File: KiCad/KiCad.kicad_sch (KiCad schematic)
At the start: 7 parts, among them J1 LDR, J2 Custom AMUX, J3 Moist Meter, J4 OLED, J5 Servo, U1 NodeMCU1.0(ESP-12E)

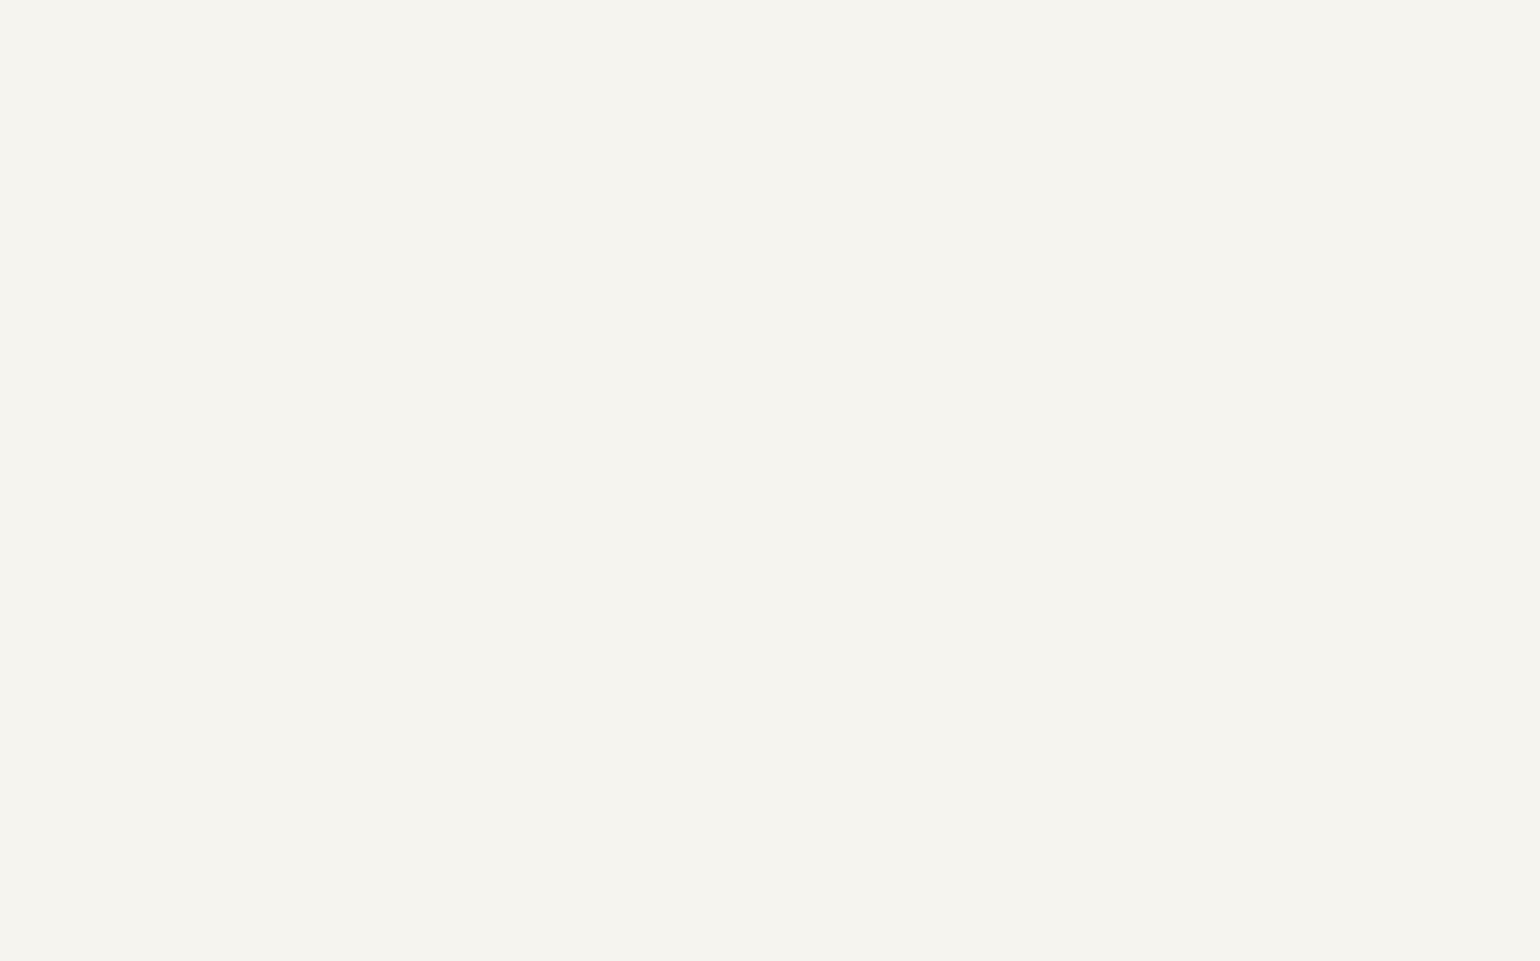
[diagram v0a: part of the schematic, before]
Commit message: kicad
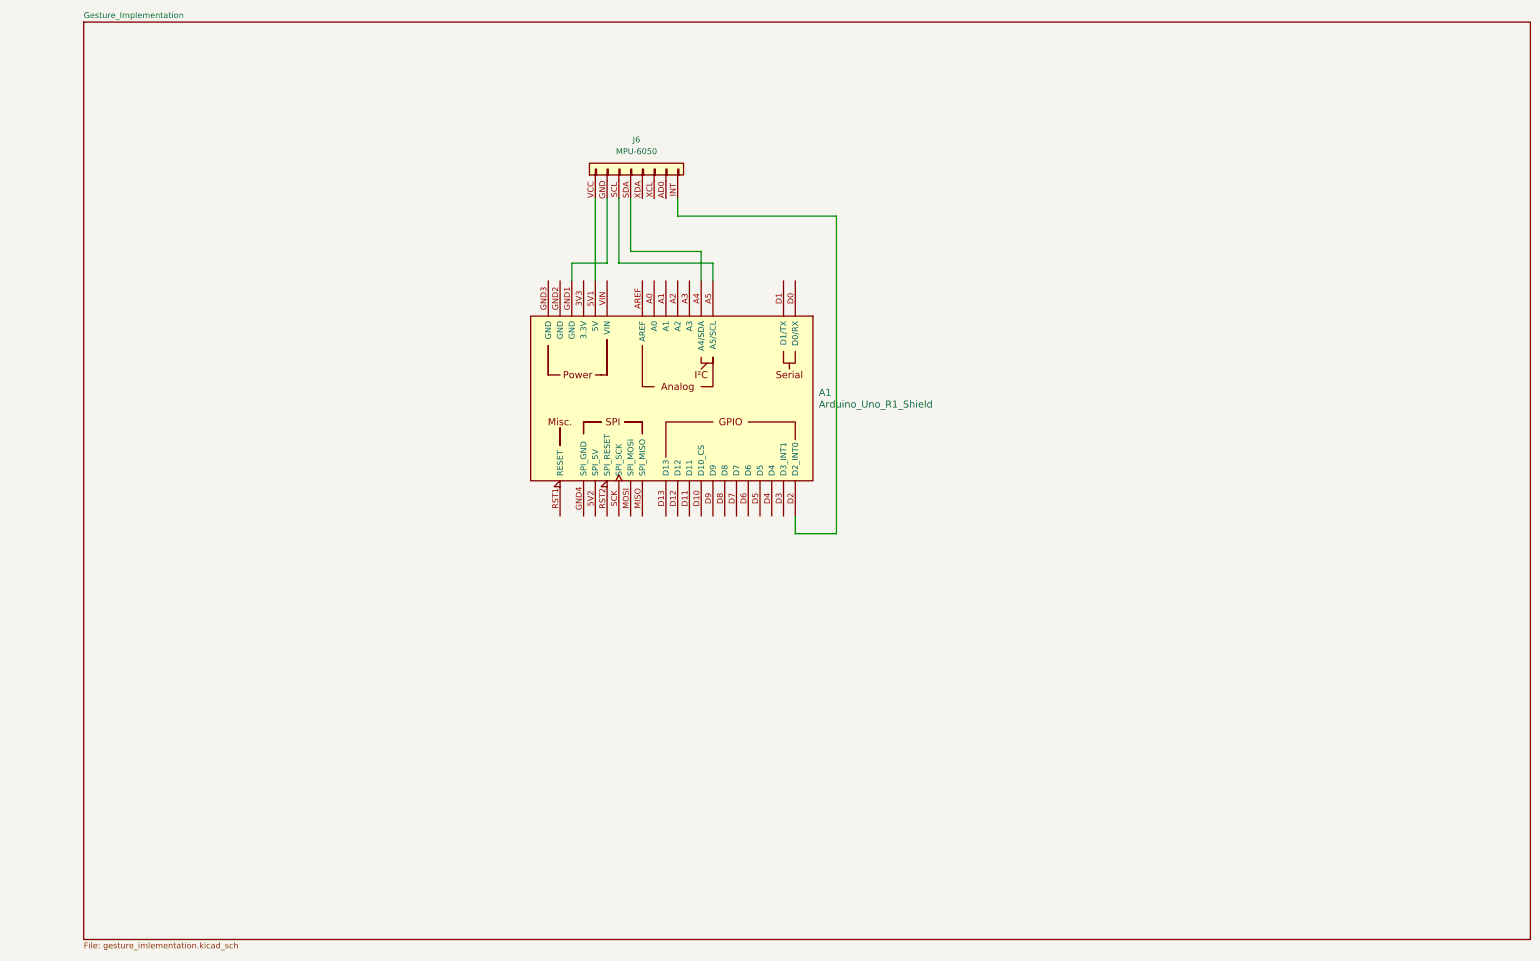
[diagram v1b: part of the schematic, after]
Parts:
- added A1: Arduino_Uno_R1_Shield, PCM_arduino-library:Arduino_Uno_R2_Shield, symbol PCM_arduino-library:Arduino_Uno_R1_Shield
- added J6: MPU-6050, symbol mpu-6050:MPU-6050
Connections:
- new net: A1.GND1 (GND), J6.GND (Pin_2)
- new net: A1.D2 (D2_INT0), J6.INT (8)
- new net: A1.A5 (A5/SCL), J6.SCL (Pin_3)
- new net: A1.A4 (A4/SDA), J6.SDA (Pin_4)
- new net: A1.5V1 (5V), J6.VCC (Pin_1)
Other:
- added sheet Gesture_Implementation (gesture_imlementation.kicad_sch)
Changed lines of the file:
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@@
+    (stroke (width 0) (type default))
+  )
+  (wire (pts (xy 486.41 45.72) (xy 486.41 114.3))
     (stroke (width 0) (type default))
   )
@@
     (stroke (width 0) (type default))
   )
+  (wire (pts (xy 434.34 41.91) (xy 434.34 59.69))
+    (stroke (width 0) (type default))
+  )
   (wire (pts (xy 129.54 130.81) (xy 128.27 130.81))
     (stroke (width 0) (type default))
@@
     (stroke (width 0) (type default))
   )
+  (wire (pts (xy 441.96 41.91) (xy 441.96 53.34))
+    (stroke (width 0) (type default))
+  )
   (wire (pts (xy 124.46 86.36) (xy 125.73 86.36))
     (stroke (width 0) (type default))
@@
     (stroke (width 0) (type default))
   )
+  (wire (pts (xy 457.2 53.34) (xy 457.2 59.69))
+    (stroke (width 0) (type default))
+  )
+  (wire (pts (xy 477.52 114.3) (xy 477.52 110.49))
+    (stroke (width 0) (type default))
+  )
   (wire (pts (xy 111.76 146.05) (xy 111.76 147.32))
     (stroke (width 0) (type default))
@@
     (stroke (width 0) (type default))
   )
+  (wire (pts (xy 429.26 55.88) (xy 429.26 59.69))
+    (stroke (width 0) (type default))
+  )
   (wire (pts (xy 120.65 144.78) (xy 120.65 147.32))
     (stroke (width 0) (type default))
@@
     (stroke (width 0) (type default))
   )
+  (wire (pts (xy 486.41 114.3) (xy 477.52 114.3))
+    (stroke (width 0) (type default))
+  )
   (wire (pts (xy 93.98 119.38) (xy 91.44 119.38))
     (stroke (width 0) (type default))
@@
     (stroke (width 0) (type default))
   )
+  (wire (pts (xy 441.96 53.34) (xy 457.2 53.34))
+    (stroke (width 0) (type default))
+  )
+  (wire (pts (xy 452.12 41.91) (xy 452.12 45.72))
+    (stroke (width 0) (type default))
+  )
   (wire (pts (xy 95.25 106.68) (xy 95.25 119.38))
     (stroke (width 0) (type default))
@@
     (stroke (width 0) (type default))
   )
+  (wire (pts (xy 439.42 41.91) (xy 439.42 55.88))
+    (stroke (width 0) (type default))
+  )
   (wire (pts (xy 90.17 118.11) (xy 90.17 123.19))
     (stroke (width 0) (type default))
@@
     (stroke (width 0) (type default))
   )
+  (wire (pts (xy 439.42 55.88) (xy 459.74 55.88))
+    (stroke (width 0) (type default))
+  )
   (wire (pts (xy 128.27 130.81) (xy 128.27 121.92))
     (stroke (width 0) (type default))
@@
     (stroke (width 0) (type default))
   )
+  (wire (pts (xy 436.88 41.91) (xy 436.88 55.88))
+    (stroke (width 0) (type default))
+  )
   (wire (pts (xy 78.74 144.78) (xy 78.74 118.11))
     (stroke (width 0) (type default))
@@
     (stroke (width 0) (type default))
   )
+  (wire (pts (xy 452.12 45.72) (xy 486.41 45.72))
+    (stroke (width 0) (type default))
+  )
+  (wire (pts (xy 459.74 55.88) (xy 459.74 59.69))
+    (stroke (width 0) (type default))
+  )
   (wire (pts (xy 95.25 119.38) (xy 168.91 119.38))
     (stroke (width 0) (type default))
@@
   )
   (wire (pts (xy 130.81 139.7) (xy 124.46 139.7))
+    (stroke (width 0) (type default))
+  )
+  (wire (pts (xy 436.88 55.88) (xy 429.26 55.88))
     (stroke (width 0) (type default))
   )
@@
         (path "/45e9d080-3c08-4e5e-927e-011f248108ba"
           (reference "J5") (unit 1)
+        )
+      )
+    )
+  )
+  (symbol (lib_id "mpu-6050:MPU-6050") (at 441.96 36.83 90) (unit 1)
+    (in_bom yes) (on_board yes) (dnp no) (fields_autoplaced)
+    (property "Reference" "J6" (at 443.23 29.21 90)
+      (effects (font (size 1.27 1.27)))
+    )
+    (property "Value" "MPU-6050" (at 443.23 31.75 90)
+      (effects (font (size 1.27 1.27)))
+    )
+    (property "Footprint" "" (at 441.96 36.83 0)
+      (effects (font (size 1.27 1.27)) hide)
+    )
+    (property "Datasheet" "~" (at 441.96 36.83 0)
+      (effects (font (size 1.27 1.27)) hide)
+    )
+    (pin "GND")
+    (pin "AD0")
+    (pin "SDA")
+    (pin "XDA")
+    (pin "INT")
+    (pin "VCC")
+    (pin "XCL")
+    (pin "SCL")
+    (instances
+      (project "KiCad"
+        (path "/45e9d080-3c08-4e5e-927e-011f248108ba"
+          (reference "J6") (unit 1)
         )
       )
@@
         (path "/45e9d080-3c08-4e5e-927e-011f248108ba"
           (reference "J2") (unit 1)
+        )
+      )
+    )
+  )
+  (symbol (lib_id "PCM_arduino-library:Arduino_Uno_R1_Shield") (at 450.85 85.09 270) (unit 1)
+    (in_bom yes) (on_board yes) (dnp no) (fields_autoplaced)
+    (property "Reference" "A1" (at 482.6 83.82 90)
+      (effects (font (size 1.524 1.524)) (justify left))
+    )
+    (property "Value" "Arduino_Uno_R1_Shield" (at 482.6 86.36 90)
+      (effects (font (size 1.524 1.524)) (justify left))
+    )
+    (property "Footprint" "PCM_arduino-library:Arduino_Uno_R2_Shield" (at 412.75 85.09 0)
+      (effects (font (size 1.524 1.524)) hide)
+    )
+    (property "Datasheet" "https://startingelectronics.org/articles/arduino/uno-r3-r2-differences/" (at 416.56 85.09 0)
+      (effects (font (size 1.524 1.524)) hide)
+    )
+    (pin "D3")
+    (pin "GND2")
+    (pin "AREF")
+    (pin "D13")
+    (pin "D0")
+    (pin "SCK")
+    (pin "D11")
+    (pin "A0")
+    (pin "A2")
+    (pin "D1")
+    (pin "RST2")
+    (pin "MOSI")
+    (pin "A5")
+    (pin "GND1")
+    (pin "A4")
+    (pin "D4")
+    (pin "RST1")
+    (pin "D6")
+    (pin "D10")
+    (pin "D8")
+    (pin "D2")
+    (pin "A1")
+    (pin "D5")
+    (pin "5V2")
+    (pin "D12")
+    (pin "D7")
+    (pin "D9")
+    (pin "A3")
+    (pin "GND4")
+    (pin "MISO")
+    (pin "5V1")
+    (pin "VIN")
+    (pin "3V3")
+    (pin "GND3")
+    (instances
+      (project "KiCad"
+        (path "/45e9d080-3c08-4e5e-927e-011f248108ba"
+          (reference "A1") (unit 1)
         )
       )
@@
       )
     )
+  )
+  (sheet (at 323.85 3.81) (size 312.42 198.12) (fields_autoplaced)
+    (stroke (width 0.1524) (type solid))
+    (fill (color 0 0 0 0.0000))
+    (property "Sheetname" "Gesture_Implementation" (at 323.85 3.0984 0)
+      (effects (font (size 1.27 1.27)) (justify left bottom))
+    )
+    (property "Sheetfile" "gesture_imlementation.kicad_sch" (at 323.85 202.5146 0) (show_name)
+      (effects (font (size 1.27 1.27)) (justify left top))
+    )
+    (instances
+      (project "KiCad"
+        (path "/45e9d080-3c08-4e5e-927e-011f248108ba" (page "2"))
+      )
+    )
